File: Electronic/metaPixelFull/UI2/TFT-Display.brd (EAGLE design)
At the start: 160 x 100 mm, 34 parts, among them IC1 74HCT14N, IC2 74HCT14N, IC3 74HCT74N, Q1 2N3906

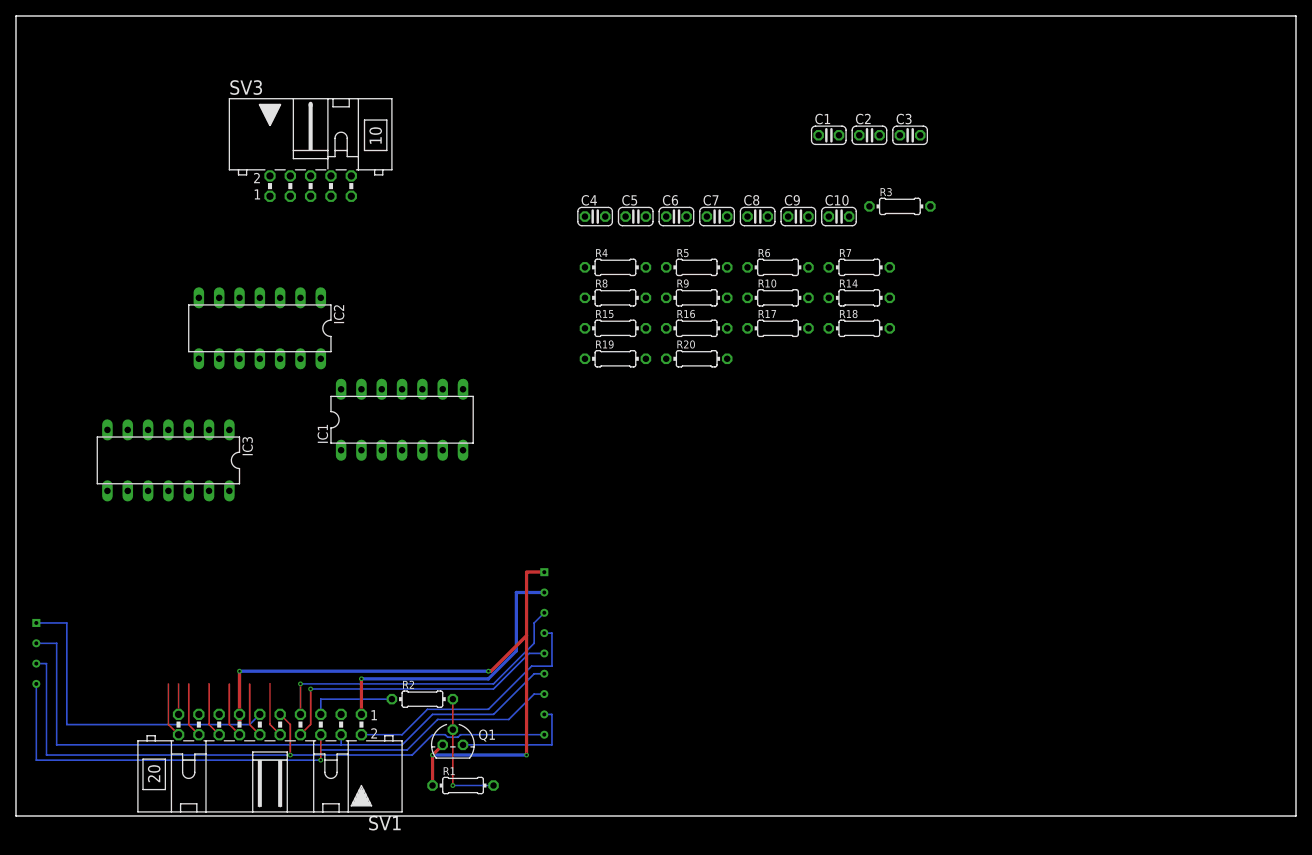
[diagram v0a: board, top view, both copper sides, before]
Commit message: Display board layout
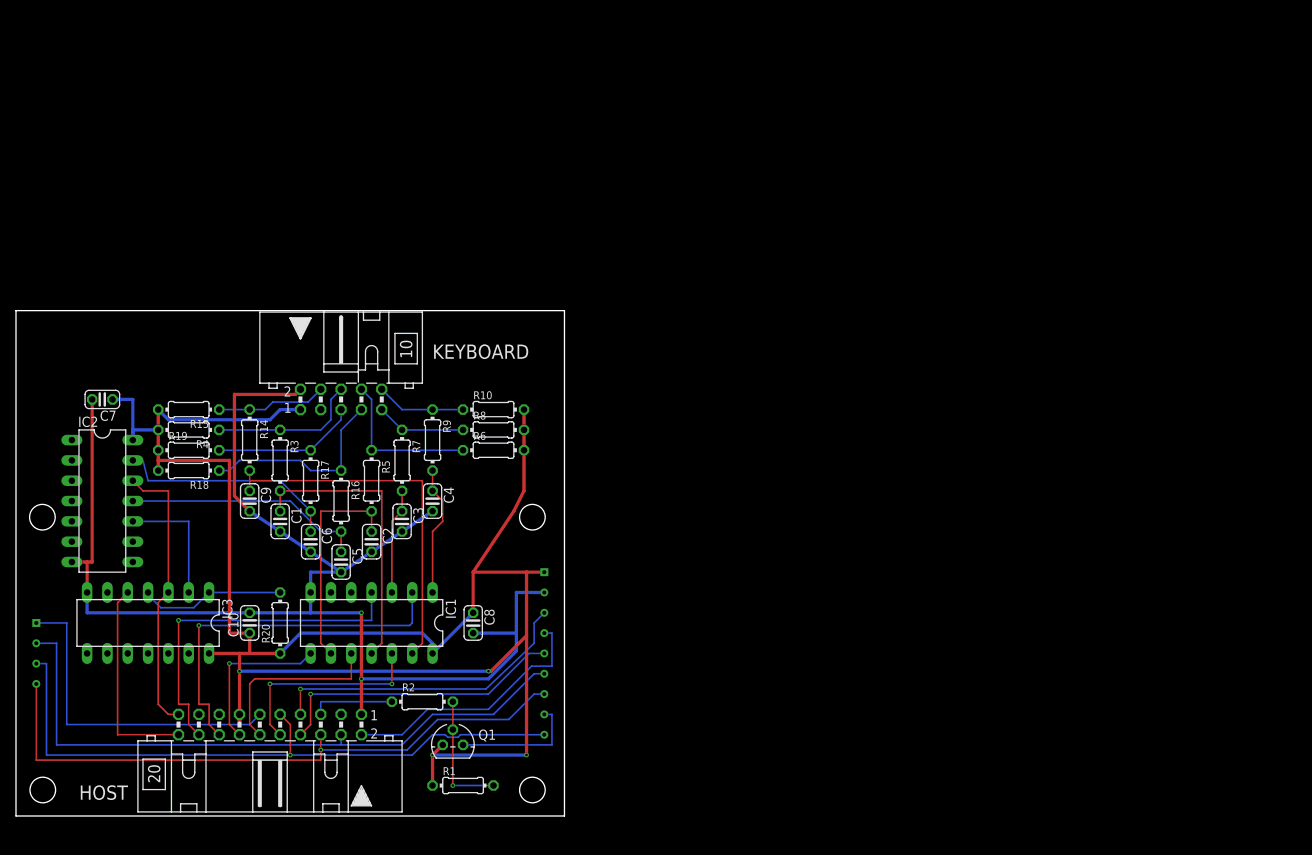
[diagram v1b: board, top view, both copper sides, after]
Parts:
- removed SV3: (no value), con-harting-ml:ML10L
- added KEYBOARD: (no value), con-harting-ml:ML10L
- HOST: value HOST -> (none)
- moved C10 89.5 mm to (29.2, 24.1), turned to 90 degrees
- moved R18 85.7 mm to (21.6, 43.2), turned to 180 degrees
- moved C1 83.9 mm to (33.0, 36.8), turned to 270 degrees
- moved R3 83.7 mm to (33.0, 44.5), turned to 270 degrees
- moved C2 80.3 mm to (44.5, 34.3), turned to 270 degrees
- moved C7 80.2 mm to (10.8, 52.1), turned to 180 degrees
- moved C3 79.8 mm to (48.3, 36.8), turned to 270 degrees
- moved R14 78.2 mm to (29.2, 47.0), turned to 270 degrees
- moved C9 77.3 mm to (29.2, 39.4), turned to 270 degrees
- moved R7 62.0 mm to (48.3, 44.5), turned to 270 degrees
- moved C8 62.0 mm to (57.1, 24.1), turned to 270 degrees
- moved R20 61.7 mm to (33.0, 24.1), turned to 90 degrees
- moved R17 61.4 mm to (36.8, 41.9), turned to 270 degrees
- moved C6 61.2 mm to (36.8, 34.3), turned to 270 degrees
- moved R4 57.1 mm to (21.6, 48.3), turned to 180 degrees
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- renumbered SV1 to HOST
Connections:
- net +3.3V: now also KEYBOARD.1; no longer SV3.1
- net ENC_1: now also KEYBOARD.7; no longer SV3.7
- net ENC_2: now also KEYBOARD.5; no longer SV3.5
- net ENC_DIR: now also HOST.20; no longer HOST.19
- net ENC_STEP: now also HOST.19; no longer HOST.20
- net GND: now also KEYBOARD.2; no longer SV3.2
- net K_1: now also KEYBOARD.4; no longer SV3.4
- net K_2: now also KEYBOARD.6; no longer SV3.6
- net K_3: now also KEYBOARD.8; no longer SV3.8
- net K_4: now also KEYBOARD.10; no longer SV3.10
- net K_5: now also KEYBOARD.9; no longer SV3.9
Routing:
- net +3.3V: track 86.2 -> 234.4 mm
- net GND: track 36.1 -> 173.5 mm, vias 1 -> 2
- net K1: track 0.00 -> 46.2 mm
- net KEY_4: track 6.88 -> 46.1 mm, vias 0 -> 1
- net KEY_5: track 6.88 -> 43.7 mm, vias 0 -> 1
- net K2: track 0.00 -> 36.1 mm
- net ENC1: track 0.00 -> 30.2 mm
- net ENC_STEP: track 6.88 -> 35.2 mm
- net ENC2: track 0.00 -> 28.3 mm
- net K3: track 0.00 -> 27.2 mm
- net ENC_1: track 0.00 -> 25.0 mm
- net ENC_DIR: track 3.81 -> 25.9 mm
- net K_3: track 0.00 -> 19.6 mm
- net KEY_1: track 6.88 -> 25.9 mm, vias 0 -> 2
- net K_2: track 0.00 -> 18.8 mm
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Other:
- board size 160 x 100 mm -> 68.6 x 63.2 mm

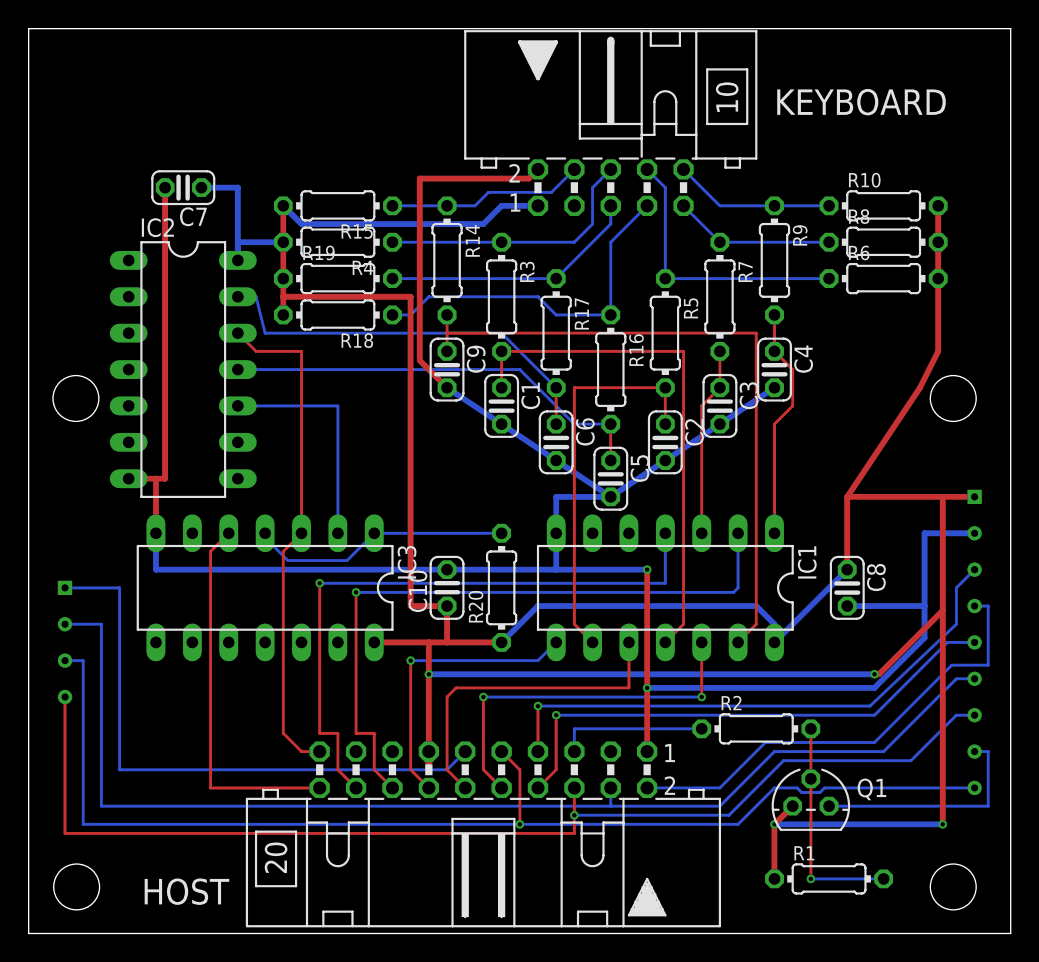
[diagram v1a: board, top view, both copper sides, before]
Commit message: The first 3 Boards are ready
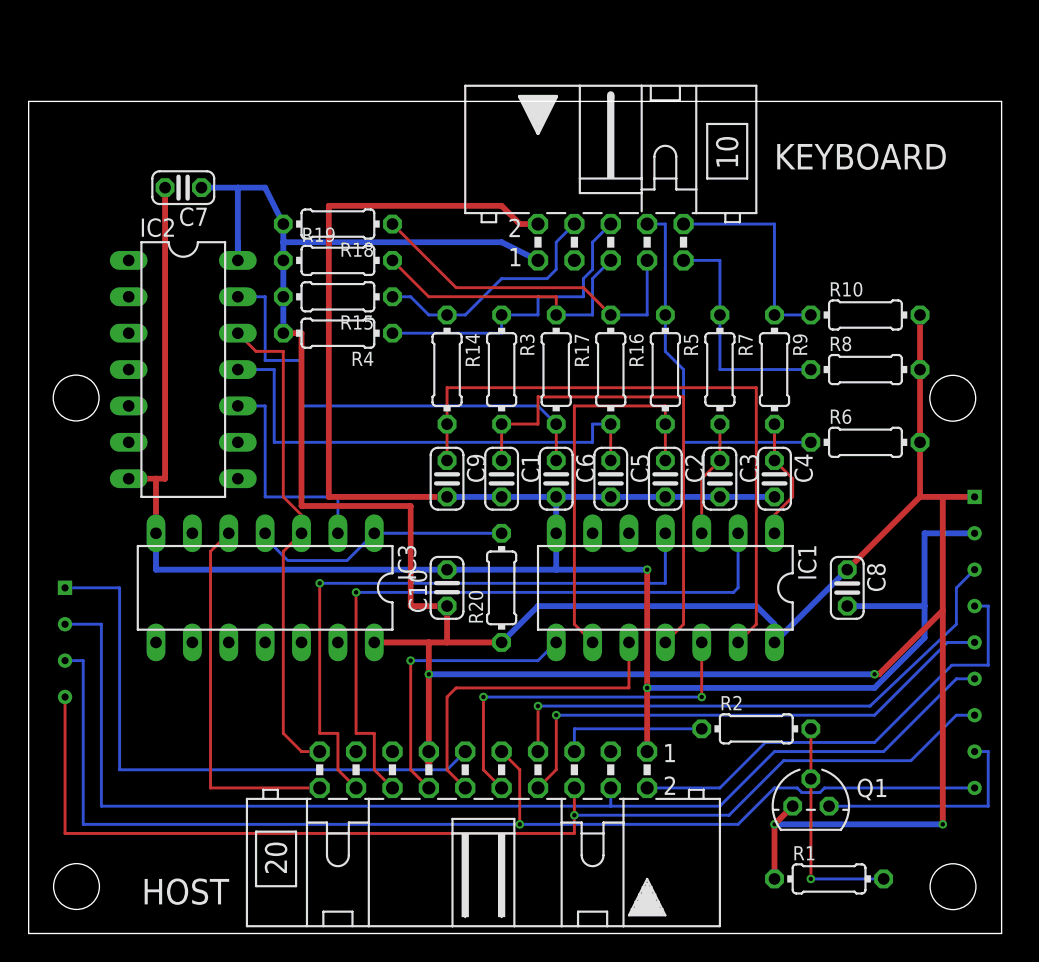
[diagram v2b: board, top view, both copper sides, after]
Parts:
- moved R6 11.5 mm to (58.4, 34.3)
- moved R8 8.98 mm to (58.4, 39.4)
- moved R10 7.73 mm to (58.4, 43.2)
- moved R14 7.62 mm to (29.2, 39.4)
- moved R9 7.62 mm to (52.1, 39.4)
- moved C4 7.62 mm to (52.1, 31.8)
- moved C9 7.62 mm to (29.2, 31.8)
- moved R18 6.35 mm to (21.6, 49.5)
- moved R4 6.35 mm to (21.6, 41.9)
- moved R15 6.35 mm to (21.6, 44.5)
- moved R3 5.08 mm to (33.0, 39.4)
- moved R7 5.08 mm to (48.3, 39.4)
- moved C1 5.08 mm to (33.0, 31.8)
- moved C3 5.08 mm to (48.3, 31.8)
- moved KEYBOARD 3.81 mm to (40.6, 48.3)
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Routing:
- net +3.3V: track 234.4 -> 220.2 mm
- net GND: track 173.5 -> 184.9 mm
- net K5: track 16.3 -> 8.67 mm
- net K_3: track 19.6 -> 25.9 mm
- net K_5: track 11.2 -> 16.5 mm
- net K4: track 13.2 -> 8.15 mm
- net ENC1: track 30.2 -> 34.9 mm
- net ENC2: track 28.3 -> 32.9 mm
- net K_4: track 11.2 -> 15.2 mm
- net K_1: track 13.8 -> 17.0 mm
- net K_2: track 18.8 -> 21.7 mm
- net ENC_2: track 18.1 -> 20.6 mm
- net K2: track 36.1 -> 34.8 mm
- net K1: track 46.2 -> 45.0 mm
- net ENC_STEP: track 35.2 -> 34.5 mm
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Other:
- board size 68.6 x 63.2 mm -> 67.9 x 58.1 mm
